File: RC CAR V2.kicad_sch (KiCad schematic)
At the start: 61 parts, among them J2 IR1, J3 IR2, J5 US, J6 LW, J7 RW, Q1 S8050, Q2 S8050, SW1 EN, SW2 BOOT, U1 L7805, U2 SRV05-4, U3 AMS1117-3.3, U4 CH340K, U6 L293DD, U7 ESP32-WROOM-32D

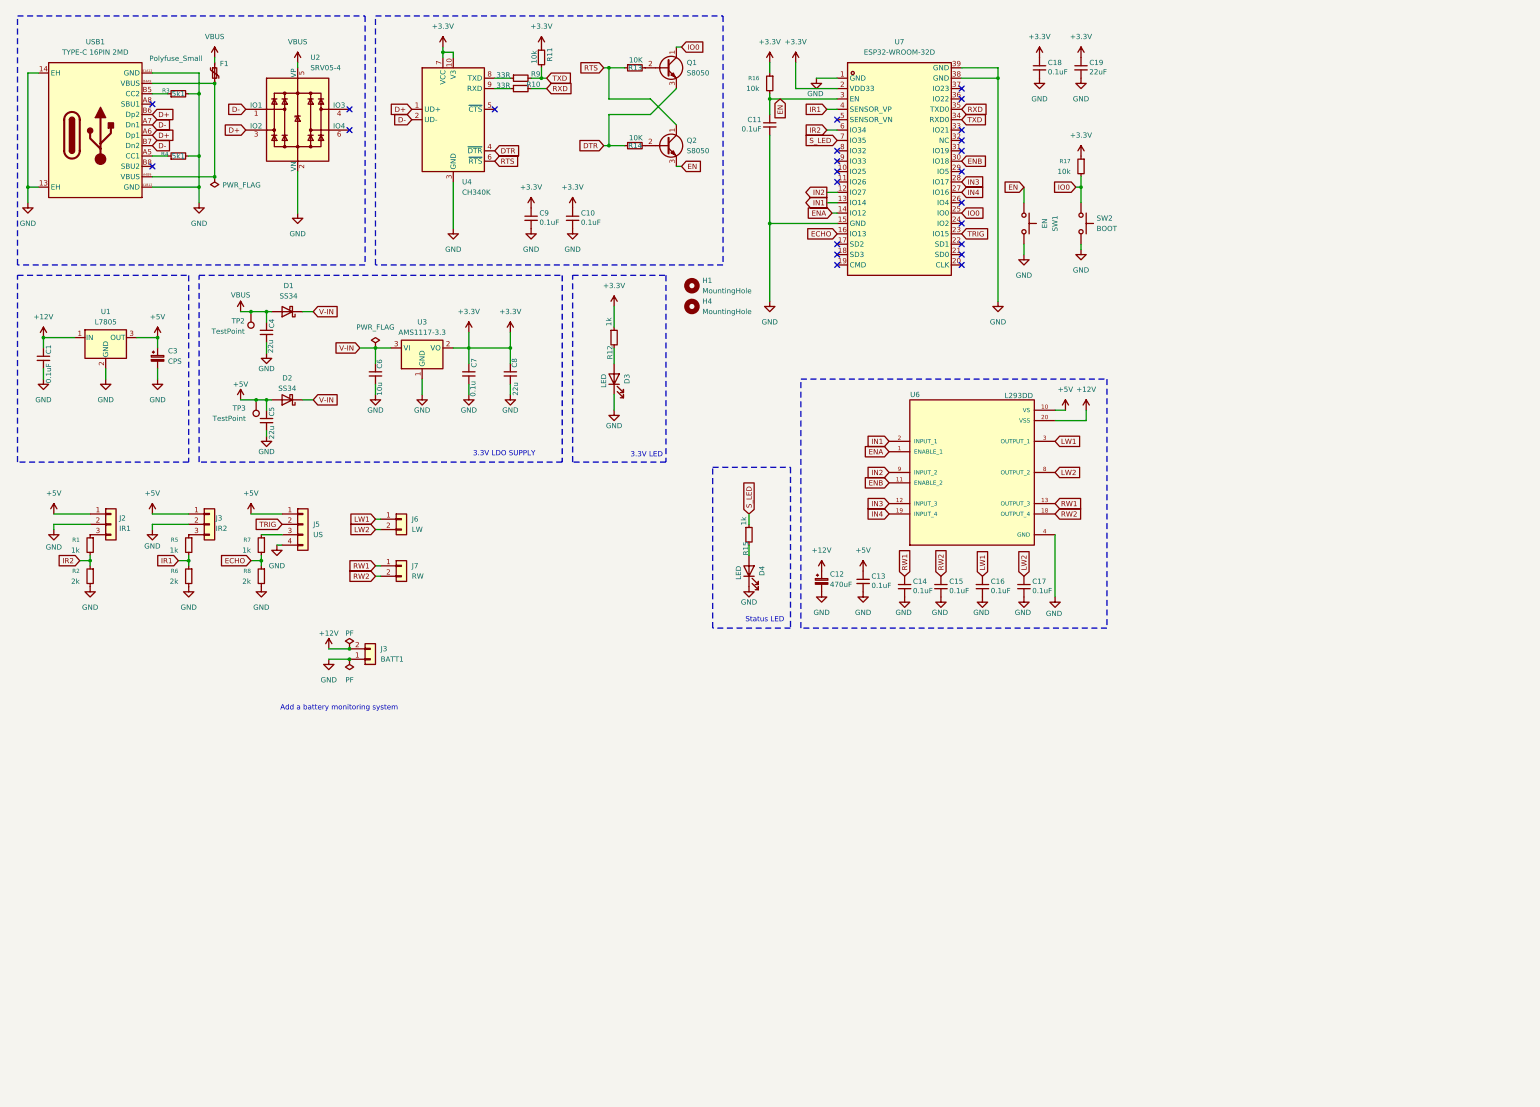
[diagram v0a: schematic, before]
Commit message: Version of the RC_CAR Circuit Routing Done
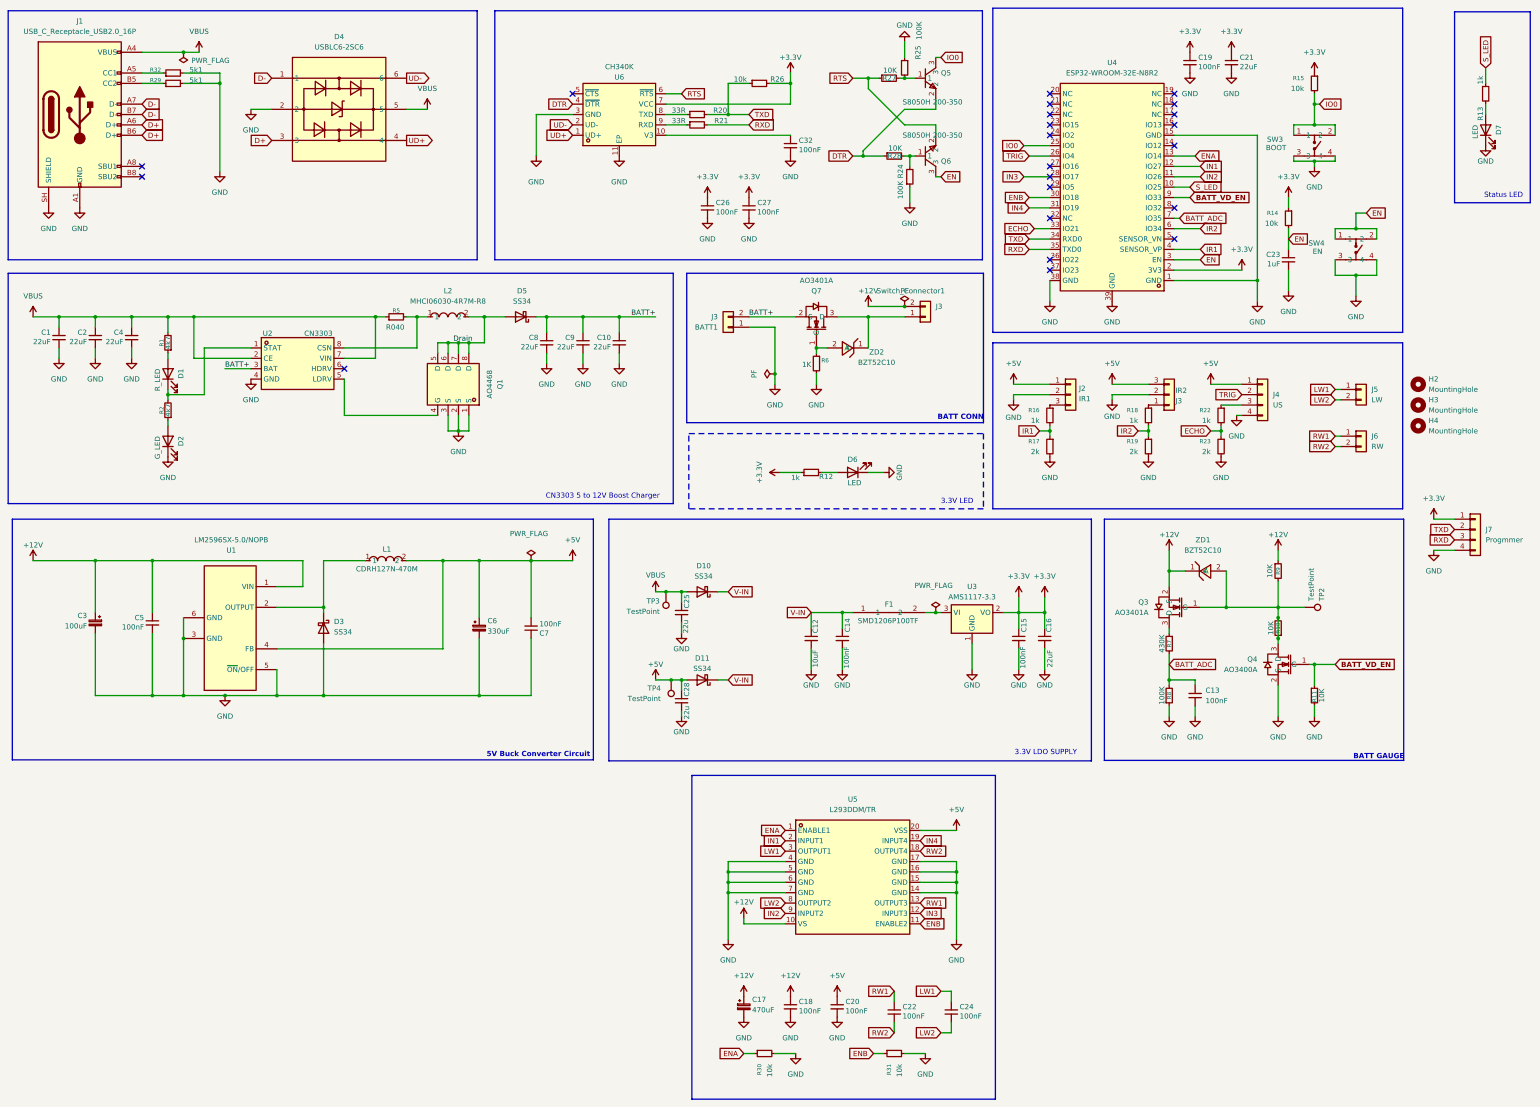
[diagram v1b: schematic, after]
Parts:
- removed C11, C15, C16: 0.1uF, Capacitor_SMD:C_0805_2012Metric_Pad1.18x1.45mm_HandSolder, symbol Device:C_Small
- removed D1, D2: SS34, Diode_SMD:D_SMA_Handsoldering, symbol Device:D_Schottky
- removed F1: Polyfuse_Small, Fuse:Fuse_0805_2012Metric_Pad1.15x1.40mm_HandSolder, symbol Device:Polyfuse_Small
- removed H1: MountingHole, MountingHole:MountingHole_2.1mm, symbol Mechanical:MountingHole
- removed Q1, Q2: S8050, Package_TO_SOT_SMD:SOT-23, symbol Transistor_BJT:BC547
- removed R16, R17: 10k, Resistor_SMD:R_0805_2012Metric_Pad1.20x1.40mm_HandSolder, symbol Device:R_Small
- removed R3, R4: 5k1, Resistor_SMD:R_0805_2012Metric_Pad1.20x1.40mm_HandSolder, symbol Device:R_Small
- removed SW1: EN, Button_Switch_SMD:SW_Tactile_SPST_NO_Straight_CK_PTS636Sx25SMTRLFS, symbol Switch:SW_Push
- removed SW2: BOOT, Button_Switch_SMD:SW_Tactile_SPST_NO_Straight_CK_PTS636Sx25SMTRLFS, symbol Switch:SW_Push
- removed U1: L7805, Package_TO_SOT_SMD:TO-263-3_TabPin2, symbol Regulator_Linear:L7805
- removed U2: SRV05-4, Package_TO_SOT_SMD:SOT-23-6, symbol Power_Protection:SRV05-4
- removed U4: CH340K, Package_SO:SSOP-10-1EP_3.9x4.9mm_P1mm_EP2.1x3.3mm, symbol Interface_USB:CH340K
- removed U6: L293DD, Package_SO:SOIC-20W_7.5x12.8mm_P1.27mm, symbol L293DD:L293DD
- removed U7: ESP32-WROOM-32D, EasyEDA:WIFIM-SMD_39P-L25.5-W18.0-P1.27-BL, symbol EasyEDA:ESP32-WROOM-32D
- removed USB1: TYPE-C 16PIN 2MD, EasyEDA:USB-C-SMD_TYPE-C-16PIN-2MD-073, symbol EasyEDA:TYPE-C16PIN2MD
- added C10, C2, C8, C9: 22uF, Capacitor_SMD:C_0805_2012Metric_Pad1.18x1.45mm_HandSolder, symbol Device:C_Small
- added C13, C14, C18, C32, C7: 100nF, Capacitor_SMD:C_0805_2012Metric_Pad1.18x1.45mm_HandSolder, symbol Device:C_Small
- added C23: 1uF, Capacitor_SMD:C_0805_2012Metric_Pad1.18x1.45mm_HandSolder, symbol Device:C_Small
- added C25, C28: 22u, Capacitor_SMD:C_0805_2012Metric_Pad1.18x1.45mm_HandSolder, symbol Device:C_Small
- added C6: 330uF, Capacitor_SMD:CP_Elec_10x10.5, symbol Device:C_Polarized_Small
- added D1: R_LED, LED_SMD:LED_0805_2012Metric_Pad1.15x1.40mm_HandSolder, symbol Device:LED
- added D10, D11: SS34, Diode_SMD:D_SMA_Handsoldering, symbol Device:D_Schottky
- added D2: G_LED, LED_SMD:LED_0805_2012Metric_Pad1.15x1.40mm_HandSolder, symbol Device:LED
- added D3, D5: SS34, Diode_SMD:D_SMA, symbol Diode:SS34
- added D4: USBLC6-2SC6, EasyEDA:SOT-23-6_L2.9-W1.6-P0.95-LS2.8-BL, symbol EasyEDA:USBLC6-2SC6
- added F1: SMD1206P100TF, EasyEDA:F1206, symbol EasyEDA:SMD1206P100TF
- added H3, H4: MountingHole, MountingHole:MountingHole_2.1mm, symbol Mechanical:MountingHole
- added J1: USB_C_Receptacle_USB2.0_16P, USB_C_Receptacle_Palconn_UTC16-G, symbol Connector:USB_C_Receptacle_USB2.0_16P
- added J7: Progmmer, Connector_PinHeader_2.54mm:PinHeader_1x04_P2.54mm_Vertical, symbol Connector_Generic:Conn_01x04
- added L1: CDRH127N-470M, EasyEDA:IND-SMD_L12.3-W12.3, symbol EasyEDA:CDRH127N-470M
- added L2: MHCI06030-4R7M-R8, EasyEDA:IND-SMD_L7.3-W6.6_MHCI06030, symbol EasyEDA:MHCI06030-4R7M-R8
- added Q1: AO4468, EasyEDA:SOP-8_L4.9-W3.9-P1.27-LS6.0-BL, symbol EasyEDA:AO4468
- added Q3, Q7: AO3401A, EasyEDA:SOT-23-3_L2.9-W1.3-P1.90-LS2.4-BR, symbol EasyEDA:AO3400A
- added Q4: AO3400A, EasyEDA:SOT-23-3_L2.9-W1.3-P1.90-LS2.4-BR, symbol EasyEDA:AO3400A
- added Q5, Q6: S8050H 200-350, EasyEDA:SOT-23-3_L2.9-W1.6-P1.90-LS2.8-BR, symbol EasyEDA:S8050H200-350
- added R1, R2: 4k7, Resistor_SMD:R_0805_2012Metric_Pad1.20x1.40mm_HandSolder, symbol Device:R_Small
- added R14, R15, R26, R30, R31: 10k, Resistor_SMD:R_0805_2012Metric_Pad1.20x1.40mm_HandSolder, symbol Device:R_Small
- added R20, R21: 33R, Resistor_SMD:R_0805_2012Metric_Pad1.20x1.40mm_HandSolder, symbol Device:R_Small
- added R24, R25, R8: 100K, Resistor_SMD:R_0805_2012Metric_Pad1.20x1.40mm_HandSolder, symbol Device:R_Small
- added R29, R32: 5k1, Resistor_SMD:R_0805_2012Metric_Pad1.20x1.40mm_HandSolder, symbol Device:R_Small
- added R5: R040, Resistor_SMD:R_1206_3216Metric_Pad1.30x1.75mm_HandSolder, symbol Device:R_Small
- added R6: 1K, Resistor_SMD:R_0805_2012Metric_Pad1.20x1.40mm_HandSolder, symbol Device:R_Small
- added R7: 430K, Resistor_SMD:R_0805_2012Metric_Pad1.20x1.40mm_HandSolder, symbol Device:R_Small
- added SW3: BOOT, EasyEDA:SW-SMD_4P-L4.2-W3.4-P2.15-LS5.2, symbol EasyEDA:HX3X4X2.5-PA-4NPUSHBUTTONSWITCH
- added SW4: EN, EasyEDA:SW-SMD_4P-L4.2-W3.4-P2.15-LS5.2, symbol EasyEDA:HX3X4X2.5-PA-4NPUSHBUTTONSWITCH
- added Switch_Connector1: J3, Connector_JST:JST_XH_B2B-XH-AM_1x02_P2.50mm_Vertical, symbol Connector_Generic:Conn_01x02
- added TP4: TestPoint, TestPoint:TestPoint_Pad_D1.0mm, symbol Connector:TestPoint
- added U1: LM2596SX-5.0/NOPB, EasyEDA:TO-263-5_L10.2-W8.9-P1.70-TL, symbol EasyEDA:LM2596SX-5.0_NOPB
- added U2: CN3303, EasyEDA:SOP-8_L4.9-W3.9-P1.27-LS6.0-BL-1, symbol EasyEDA:CN3303
- added U4: ESP32-WROOM-32E-N8R2, EasyEDA:WIFI-SMD_ESP32-WROOM-32E, symbol EasyEDA:ESP32-WROOM-32E-N8R2
- added U5: L293DDM/TR, EasyEDA:SOP-20_L12.8-W7.5-P1.27-LS10.4-BL, symbol EasyEDA:L293DDM_TR
- added U6: CH340K, EasyEDA:ESOP-10_L4.9-W3.9-P1.00-LS6.2-BL-EP, symbol EasyEDA:CH340K
- added ZD1, ZD2: BZT52C10, EasyEDA:SOD-123_L2.8-W1.8-LS3.7-RD, symbol EasyEDA:BZT52C10
- C1: value 0.1uF -> 22uF
- C12: renamed from C6; value 10u -> 10uF
- C15: renamed from C7; value 0.1u -> 100nF
- C16: renamed from C8; value 22u -> 22uF
- C17: renamed from C12; footprint Capacitor_THT:CP_Radial_D8.0mm_P3.50mm -> Capacitor_SMD:C_Elec_10x10.2
- C19: renamed from C18; value 0.1uF -> 100nF
- C20: renamed from C13; value 0.1uF -> 100nF
- C22: renamed from C14; value 0.1uF -> 100nF
- C24: renamed from C17; value 0.1uF -> 100nF
- C26: renamed from C9; value 0.1uF -> 100nF
- C27: renamed from C10; value 0.1uF -> 100nF
- C3: value CPS -> 100uF; footprint Capacitor_THT:CP_Radial_D5.0mm_P2.50mm -> Capacitor_SMD:CP_Elec_8x10; LCSC Part (none) -> C3352
- C4: value 22u -> 22uF
- C5: value 22u -> 100nF; LCSC Part (none) -> C1711
- R10, R9: value 33R -> 10K
- R11: value 10k -> 10K
- TP2: footprint TestPoint:TestPoint_Pad_D1.0mm -> TestPoint:TestPoint_Pad_1.0x1.0mm
- renumbered C19 to C21, D3 to D6, D4 to D7, H4 to H2, J5 to J4, J6 to J5, J7 to J6, R15 to R13, R1 to R16, R2 to R17, R5 to R18, R6 to R19, R7 to R22, R8 to R23, R13 to R27, R14 to R28
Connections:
- net +12V: now also C3.1, C5.1, R9.1, C18.1, Q3.2 (S), Switch_Connector1.2 (Pin_2), U1.1 (VIN), U5.10 (VS), ZD1.1 (K); no longer BATT1.2 (Pin_2), C1.1
- net +3.3V: now also J7.1 (Pin_1), R14.1, R15.1, R26.2, U4.2 (3V3), U6.7 (VCC); no longer R11.1
- net +5V: now also J3.3 (Pin_3), C28.1, C6.1, C7.2, D11.2 (A), L1.2, TP4.1, U1.4 (FB), U5.20 (VSS); no longer C3.1, C5.1, J3.1 (Pin_1), TP3.1
- net D+: now also D4.3, J1.A6 (D+), J1.B6 (D+)
- net D-: now also D4.1, J1.A7 (D-), J1.B7 (D-)
- net DTR: now also Q5.2, U6.4 (~{DTR})
- net ECHO: now also U4.33 (IO21)
- net EN: now also C23.1, Q6.3, R14.2, SW4.1, SW4.2, U4.3 (EN)
- net ENA: now also R30.1, U4.13 (IO14), U5.1 (ENABLE1)
- net ENB: now also R31.1, U4.30 (IO18), U5.11 (ENABLE2)
- net GND: now also R11.2, C10.2, C13.2, C14.2, C18.2, C2.2, C23.2, C25.2, C28.2, C32.2, C6.2, C7.1, C8.2, C9.2, D2.1 (K), D3.2 (A), D4.2, J1.A1 (GND), J1.A12 (GND), J1.B1 (GND), J1.B12 (GND), J1.SH (SHIELD), J7.4 (Pin_4), Q1.1 (S), Q1.2 (S), Q1.3 (S), Q4.2 (S), R24.1, R25.1, R29.2, R30.2, R31.2, R32.2, R6.2, R8.1, SW3.3, SW3.4, SW4.3, SW4.4, U1.3 (GND), U1.5 (~{ON}/OFF), U1.6 (GND), U2.4 (GND), U4.1 (GND), U4.15 (GND), U4.38 (GND), U4.39 (GND), U5.14 (GND), U5.15 (GND), U5.16 (GND), U5.17 (GND), U5.4 (GND), U5.5 (GND), U5.6 (GND), U5.7 (GND), U6.11 (EP), U6.3 (GND); no longer C22.2, C24.2
- net IN1: now also U4.12 (IO27), U5.2 (INPUT1)
- net IN2: now also U4.11 (IO26), U5.9 (INPUT2)
- net IN3: now also U4.28 (IO17), U5.12 (INPUT3)
- net IN4: now also U4.31 (IO19), U5.19 (INPUT4)
- net IO0: now also Q5.3, R15.2, SW3.1, SW3.2, U4.25 (IO0)
- net IR1: now also R16.2, R17.1, U4.4 (SENSOR_VP); no longer R18.2, R19.1
- net IR2: now also R18.2, R19.1, U4.6 (IO34); no longer R16.2, R17.1
- net LW1: now also C24.1, U5.3 (OUTPUT1)
- net LW2: now also C24.2, U5.8 (OUTPUT2); no longer C24.1
- net RTS: now also Q6.2, U6.6 (~{RTS})
- net RW1: now also U5.13 (OUTPUT3)
- net RW2: now also C22.2, U5.18 (OUTPUT4)
- net RXD: now also J7.3 (Pin_3), R21.2, U4.35 (TXD0); no longer R10.2
- net S_LED: now also U4.10 (IO25)
- net TRIG: now also U4.26 (IO4)
- net TXD: now also J7.2 (Pin_2), R20.2, R26.1, U4.34 (RXD0); no longer R11.2, R9.2
- net V-IN: now also C14.1, D10.1 (K), D11.1 (K), F1.1; no longer U3.3 (VI)
- net VBUS: now also C1.1, TP3.1, C2.1, C25.1, D10.2 (A), D4.5, J1.A4 (VBUS), J1.A9 (VBUS), J1.B4 (VBUS), J1.B9 (VBUS), R1.2, R5.1, U2.2 (CE), U2.7 (VIN); no longer TP2.1
- net at R18.1: now also J3.1 (Pin_1); no longer J3.3 (Pin_3)
- net at R10.1: now also R10.2, R9.2, TP2.1, Q3.1 (G), Q4.3 (D), ZD1.2 (A)
- net at R27.2: now also Q5.1, R25.2
- net at R28.2: now also Q6.1, R24.2
- new net: C32.1, U6.10 (V3)
- new net: R20.1, U6.8 (TXD)
- new net: R21.1, U6.9 (RXD)
- new net: Q3.3 (D), R7.1
- new net: D1.1 (K), R2.2, U2.1 (STAT)
- new net: Q1.4 (G), U2.5 (LDRV)
- new net: L2.1, R5.2, U2.8 (CSN)
- new net: D2.2 (A), R2.1
- new net: D1.2 (A), R1.1
- new net: D3.1 (K), L1.1, U1.2 (OUTPUT)
- new net: Q7.3 (D), Switch_Connector1.1 (Pin_1), ZD2.1 (K)
- new net: Q7.1 (G), R6.1, ZD2.2 (A)
- new net: J1.A5 (CC1), R32.1
- new net: J1.B5 (CC2), R29.1
- new net: F1.2, U3.3 (VI)
- new net BATT+: BATT1.2 (Pin_2), C10.1, C8.1, C9.1, D5.1 (K), Q7.2 (S), U2.3 (BAT)
- new net BATT_ADC: C13.1, R7.2, R8.2, U4.7 (IO35)
- new net BATT_VD_EN: Q4.1 (G), R11.1, U4.9 (IO33)
- new net Drain: D5.2 (A), L2.2, Q1.5 (D), Q1.6 (D), Q1.7 (D), Q1.8 (D)
- new net UD+: D4.4, U6.1 (UD+)
- new net UD-: D4.6, U6.2 (UD-)
- no-connect marks 24 -> 22
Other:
- note added: "5V Buck Converter Circuit"
- note added: "BATT CONN"
- note added: "BATT GAUGE"
- note added: "CN3303 5 to 12V Boost Charger"
- note removed: "Add a battery monitoring system"
- moved on the sheet: BATT1, C12, C15, C16, C17, C19, C20, C21, C22, C24, C26, C27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
